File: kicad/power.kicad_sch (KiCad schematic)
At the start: 64 parts, among them Q3 CSD17308Q3, Q4 CSD17308Q3, Q7 CSD17308Q3, Q8 CSD17308Q3, U17 LTC3856, U3 AP3211, U4 +0V8, U5 MCP1824T-1802E, U6 MCP1824T-0802E

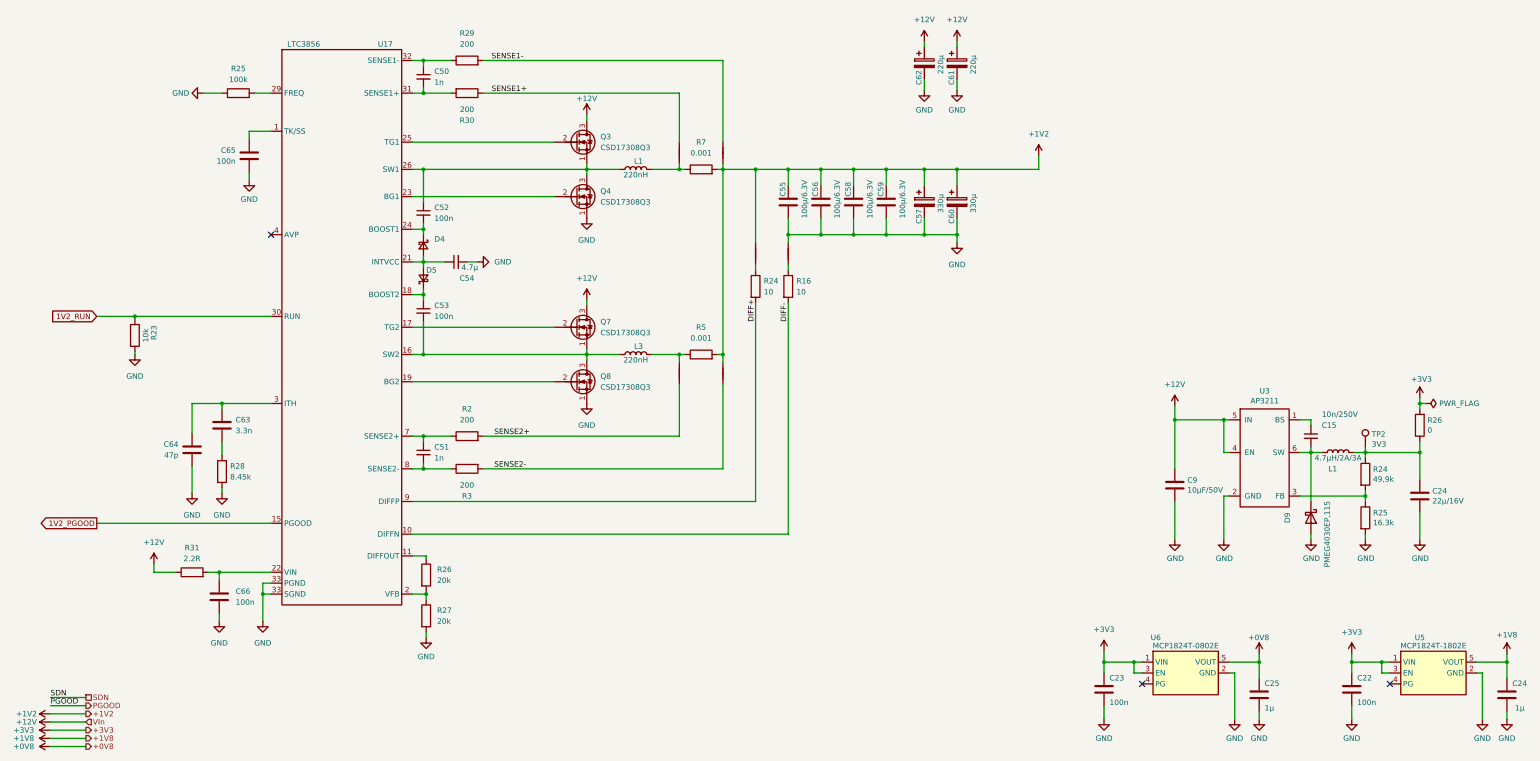
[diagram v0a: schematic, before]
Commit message: added mp8796 (wip)
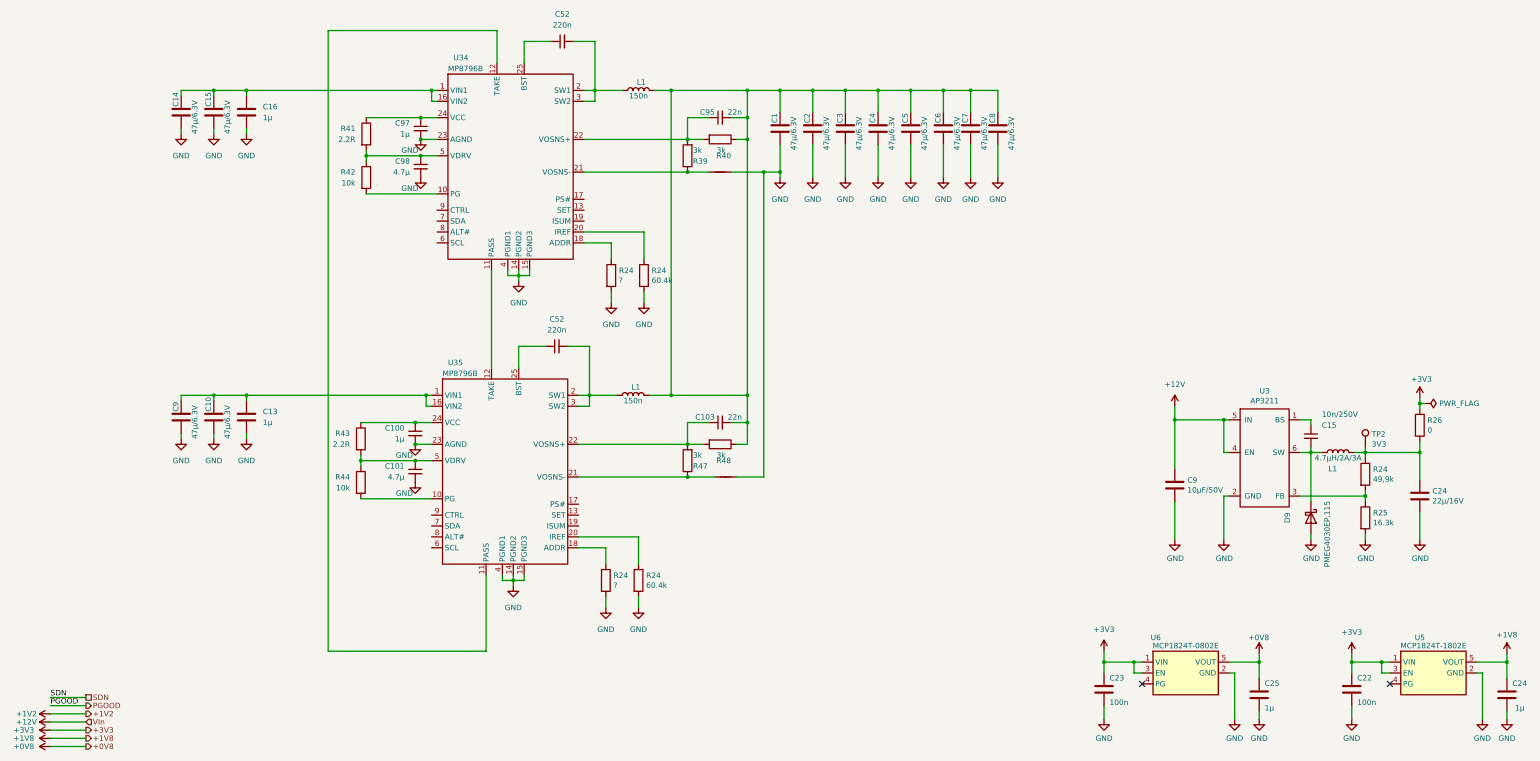
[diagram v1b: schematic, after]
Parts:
- removed C50, C51: 1n, Capacitor_SMD:C_0805_2012Metric, symbol Device:C_Small
- removed C52, C53: 100n, Capacitor_SMD:C_0805_2012Metric, symbol Device:C_Small
- removed C54: 4.7µ, Capacitor_SMD:C_0805_2012Metric, symbol Device:C_Small
- removed C55, C56, C58, C59: 100µ/6.3V, Capacitor_SMD:C_1210_3225Metric, symbol Device:C
- removed C57, C60: 330µ, Capacitor_SMD:CP_Elec_5x5.8, symbol Device:C_Polarized
- removed C61, C62: 220µ, Capacitor_SMD:CP_Elec_5x5.8, symbol Device:C_Polarized
- removed C63: 3.3n, Capacitor_SMD:C_0805_2012Metric, symbol Device:C
- removed C64: 47p, Capacitor_SMD:C_0805_2012Metric, symbol Device:C
- removed C65, C66: 100n, Capacitor_SMD:C_0805_2012Metric, symbol Device:C
- removed D4, D5: D_Schottky_Small, Diode_SMD:D_SOD-323, symbol Device:D_Schottky_Small
- removed L3: 220nH, myfootprints:IFLR-4031GC-01-8x10, symbol Device:L
- removed NT1 (x3), NT3, NT4: NetTie_2, NetTie:NetTie-2_SMD_Pad0.5mm, symbol Device:NetTie_2
- removed Q3, Q4, Q7, Q8: CSD17308Q3, Package_SON:VSONP-8-1EP_5x6_P1.27mm, symbol Device:Q_NMOS_SGD
- removed R16, R24: 10, Resistor_SMD:R_0805_2012Metric, symbol Device:R
- removed R2, R29, R3, R30: 200, Resistor_SMD:R_0805_2012Metric, symbol Device:R
- removed R23: 10k, Resistor_SMD:R_0805_2012Metric, symbol Device:R
- removed R25: 100k, Resistor_SMD:R_0805_2012Metric, symbol Device:R
- removed R26, R27: 20k, Resistor_SMD:R_0805_2012Metric, symbol Device:R
- removed R28: 8.45k, Resistor_SMD:R_0805_2012Metric, symbol Device:R
- removed R31: 2.2R, Resistor_SMD:R_2010_5025Metric, symbol Device:R
- removed R5, R7: 0.001, Resistor_SMD:R_2010_5025Metric, symbol Device:R
- removed U17: LTC3856, Package_DFN_QFN:QFN-32-1EP_5x5mm_P0.5mm_EP3.45x3.45mm_ThermalVias, symbol mylib7:LTC3856_reduced
- added C1, C10, C14, C15, C2, C3, C4, C5, C6, C7, C8, C9: 47µ/6.3V, Capacitor_SMD:C_1210_3225Metric, symbol Device:C
- added C100, C97: 1µ, Capacitor_SMD:C_0805_2012Metric, symbol Device:C_Small
- added C101, C98: 4.7µ, Capacitor_SMD:C_0805_2012Metric, symbol Device:C_Small
- added C103, C95: 22n, Capacitor_SMD:C_0805_2012Metric, symbol Device:C_Small
- added C13, C16: 1µ, Capacitor_SMD:C_0805_2012Metric, symbol Device:C
- added C52 (x2): 220n, Capacitor_SMD:C_0805_2012Metric, symbol Device:C_Small
- added L1: 150n, myfootprints:IFLR-4031GC-01-8x10, symbol Device:L
- added NT1: NetTie_2, NetTie:NetTie-2_SMD_Pad0.5mm, symbol Device:NetTie_2
- added R24 (x2): ?, Resistor_SMD:R_0805_2012Metric, symbol Device:R
- added R24 (x2): 60.4k, Resistor_SMD:R_0805_2012Metric, symbol Device:R
- added R39, R40, R47, R48: 3k, Resistor_SMD:R_0805_2012Metric, symbol Device:R
- added R41, R43: 2.2R, Resistor_SMD:R_0805_2012Metric, symbol Device:R
- added R42, R44: 10k, Resistor_SMD:R_0805_2012Metric, symbol Device:R
- added U34, U35: MP8796B, myfootprints:MP8796B, symbol mylib7:MP8796B
- L1: value 220nH -> 150n
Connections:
- net GND: now also NT2.2, C1.2, C10.2, C100.2, C101.2, C13.2, C14.2, C15.2, C16.2, C2.2, C3.2, C4.2, C5.2, C6.2, C7.2, C8.2, C9.2, C97.2, C98.2, NT1.2, R24.2, R24.2, R24.2, R24.2, U34.14 (PGND2), U34.15 (PGND3), U34.23 (AGND), U34.4 (PGND1), U35.14 (PGND2), U35.15 (PGND3), U35.23 (AGND), U35.4 (PGND1)
- net at L1.1: now also C52.2, U34.2 (SW1), U34.3 (SW2)
- net at L1.2: now also C1.1, C103.2, C2.1, C3.1, C4.1, C5.1, C6.1, C7.1, C8.1, C95.2, L1.2, R40.1, R48.1
- net SENSE2+: no longer names the net of NT2.1
- net SENSE2+: now also R39.1, U34.21 (VOSNS-)
- new net: C101.1, R43.2, R44.1, U35.5 (VDRV)
- new net: R44.2, U35.10 (PG)
- new net: C14.1, C15.1, C16.1, U34.1 (VIN1), U34.16 (VIN2)
- new net: R42.2, U34.10 (PG)
- new net: U34.11 (PASS), U35.12 (TAKE)
- new net: U34.12 (TAKE), U35.11 (PASS)
- new net: R24.1, U34.18 (ADDR)
- new net: R24.1, U34.20 (IREF)
- new net: C95.1, R39.2, R40.2, U34.22 (VOSNS+)
- new net: C97.1, R41.1, U34.24 (VCC)
- new net: C52.1, U34.25 (BST)
- new net: C98.1, R41.2, R42.1, U34.5 (VDRV)
- new net: NT1.1, R47.1, U35.21 (VOSNS-)
- new net: C103.1, R47.2, R48.2, U35.22 (VOSNS+)
- new net: C52.2, L1.1, U35.2 (SW1), U35.3 (SW2)
- new net: R24.1, U35.20 (IREF)
- new net: C52.1, U35.25 (BST)
- new net: C10.1, C13.1, C9.1, U35.1 (VIN1), U35.16 (VIN2)
- new net: R24.1, U35.18 (ADDR)
- new net: C100.1, R43.1, U35.24 (VCC)
- no-connect marks 3 -> 2
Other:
- moved on the sheet: L1
